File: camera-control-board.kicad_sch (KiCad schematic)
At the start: 24 parts, among them J1 DF12NB-36DS-0.5V_51_, J2 10104110-0001LF, J3 104031-0811, U1 STM32H743IITx, U2 IS42S32800J-7TLI, Y2 Crystal_GND2

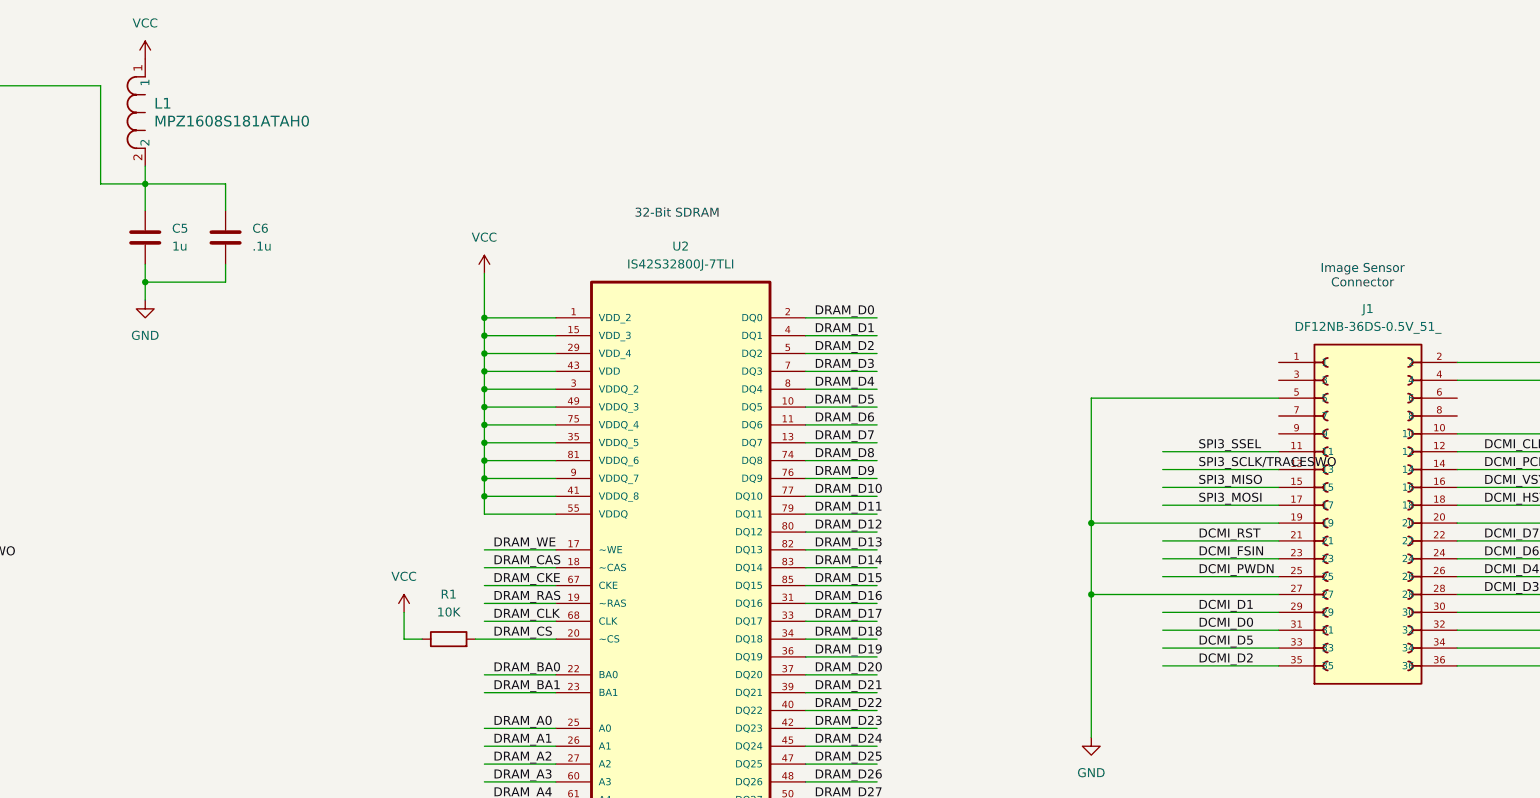
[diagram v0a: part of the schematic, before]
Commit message: configured library and repo correctly. edits incoming
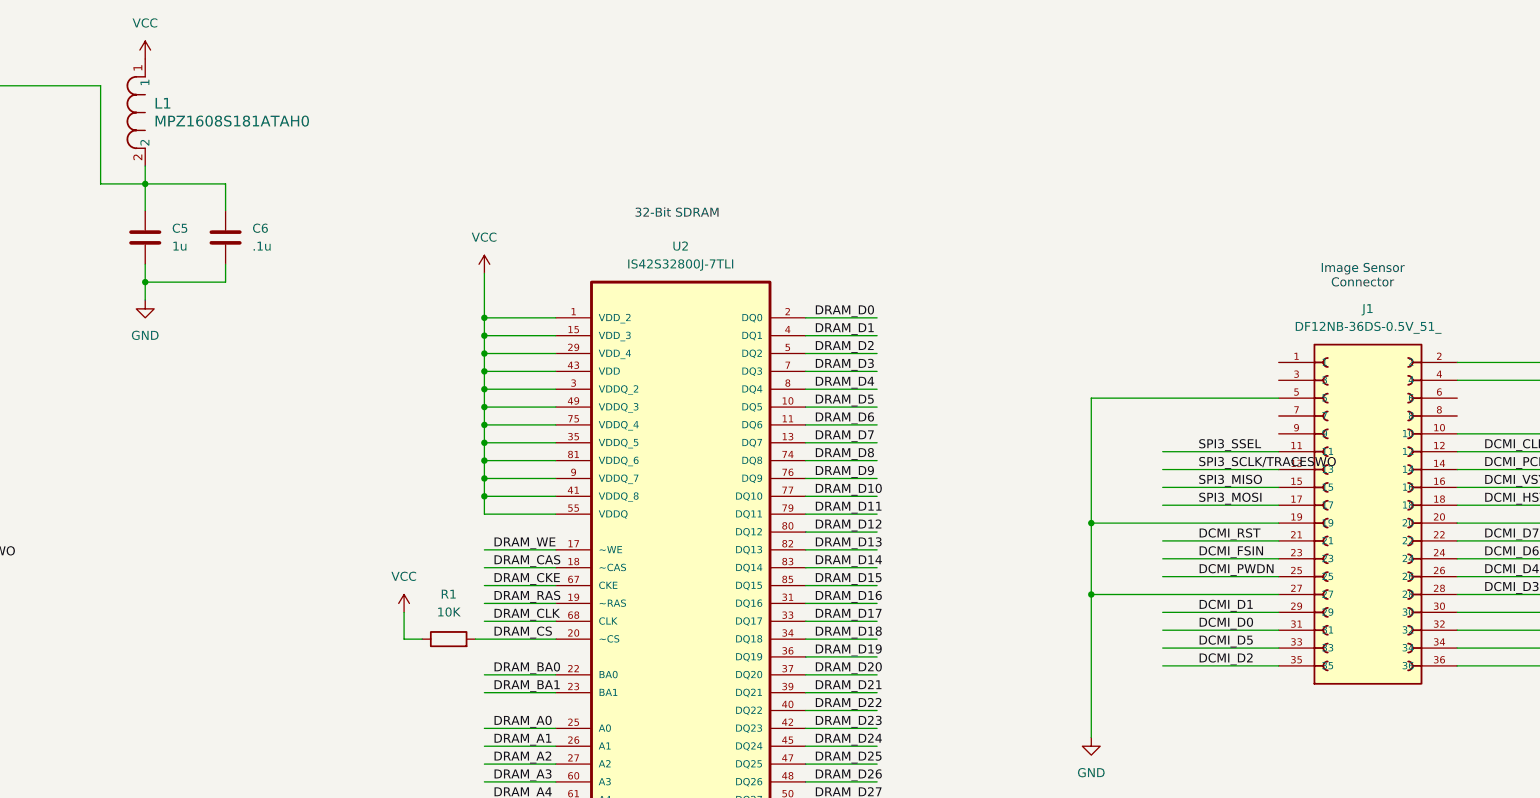
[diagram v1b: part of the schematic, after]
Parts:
- J1: symbol DF12NB-36DS-0.5V_51_:DF12NB-36DS-0.5V_51_ -> Argus_Connectors:DF12NB-36DS-0.5V_51_
- J2: symbol 10104110-0001LF:10104110-0001LF -> Argus_Connectors:10104110-0001LF
- J3: symbol 104031-0811:104031-0811 -> Argus_Connectors:104031-0811
- L1: symbol 2024-09-28_22-13-49:MPZ1608S181ATAH0 -> Argus_Misc:MPZ1608S181ATAH0
- RN1: symbol EXB-V8V103JV:EXB-V8V103JV -> Argus_Misc:EXB-V8V103JV
- U2: symbol IS42S32800J-7TLI:IS42S32800J-7TLI -> Argus_ICs:IS42S32800J-7TLI
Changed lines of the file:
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@@
 	)
 	(symbol
-		(lib_id "DF12NB-36DS-0.5V_51_:DF12NB-36DS-0.5V_51_")
+		(lib_id "Argus_Connectors:DF12NB-36DS-0.5V_51_")
 		(at 405.13 88.9 0)
 		(unit 1)
@@
 	)
 	(symbol
-		(lib_id "IS42S32800J-7TLI:IS42S32800J-7TLI")
+		(lib_id "Argus_ICs:IS42S32800J-7TLI")
 		(at 307.34 125.73 0)
 		(unit 1)
@@
 	)
 	(symbol
-		(lib_id "104031-0811:104031-0811")
+		(lib_id "Argus_Connectors:104031-0811")
 		(at 524.51 45.72 0)
 		(unit 1)
@@
 	)
 	(symbol
-		(lib_id "2024-09-28_22-13-49:MPZ1608S181ATAH0")
+		(lib_id "Argus_Misc:MPZ1608S181ATAH0")
 		(at 231.14 38.1 90)
 		(unit 1)
@@
 	)
 	(symbol
-		(lib_id "EXB-V8V103JV:EXB-V8V103JV")
+		(lib_id "Argus_Misc:EXB-V8V103JV")
 		(at 513.08 91.44 0)
 		(unit 1)
@@
 	)
 	(symbol
-		(lib_id "10104110-0001LF:10104110-0001LF")
+		(lib_id "Argus_Connectors:10104110-0001LF")
 		(at 107.95 322.58 0)
 		(unit 1)
